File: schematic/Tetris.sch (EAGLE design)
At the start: 16 parts, among them U1 ATTINY45-20P, U2 OLED_0.96_I2C, X1 Batt

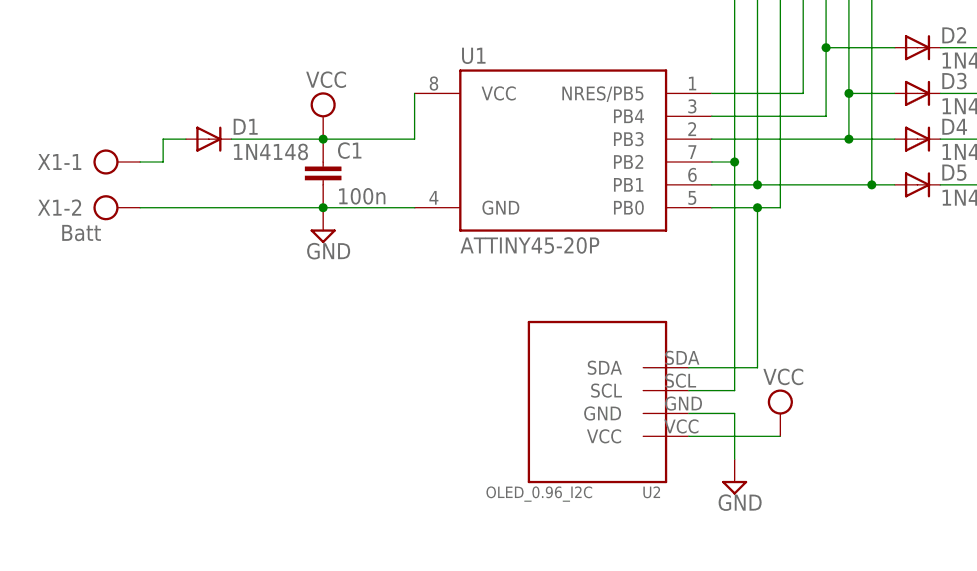
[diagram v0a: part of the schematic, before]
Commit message: Add files via upload
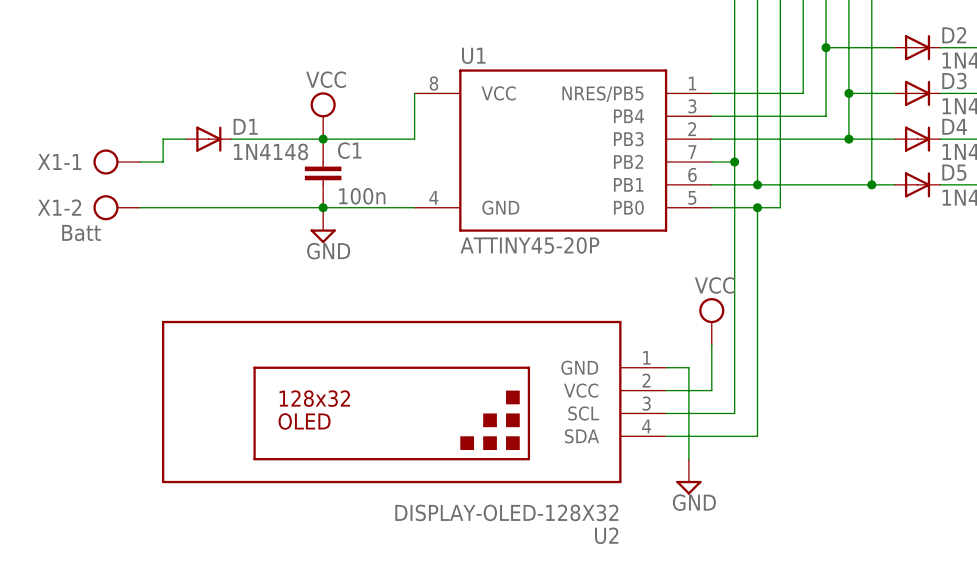
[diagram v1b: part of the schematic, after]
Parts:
- U2: value OLED_0.96_I2C -> DISPLAY-OLED-128X32; device tft_1_8_1_44_oled_0_96:OLED_0.96_I2C -> diy-modules:DISPLAY-OLED-128X32
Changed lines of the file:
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@@
 <parts>
 <part name="JP1" library="avr-7" deviceset="AVR-ISP-10" device=""/>
-<part name="U2" library="tft_1_8_1_44_oled_0_96" deviceset="OLED_0.96_I2C" device=""/>
 <part name="S1" library="switch-omron" deviceset="10-XX" device="" value="A"/>
 <part name="S2" library="switch-omron" deviceset="10-XX" device="" value="Up"/>
@@
 <part name="SUPPLY5" library="supply2" deviceset="VCC" device=""/>
 <part name="SUPPLY6" library="supply2" deviceset="VCC" device=""/>
+<part name="U2" library="diy-modules" deviceset="DISPLAY-OLED-128X32" device=""/>
 </parts>
 <sheets>
@@
 <instances>
 <instance part="JP1" gate="G$1" x="68.58" y="68.58"/>
-<instance part="U2" gate="G$1" x="68.58" y="10.16" rot="R90"/>
 <instance part="S1" gate="1" x="132.08" y="50.8" rot="R270"/>
 <instance part="S2" gate="1" x="149.86" y="50.8" rot="R270"/>
@@
 <instance part="SUPPLY1" gate="GND" x="58.42" y="58.42"/>
 <instance part="SUPPLY2" gate="GND" x="38.1" y="27.94"/>
-<instance part="SUPPLY3" gate="GND" x="83.82" y="0"/>
-<instance part="SUPPLY4" gate="G$1" x="88.9" y="7.62"/>
+<instance part="SUPPLY3" gate="GND" x="78.74" y="0"/>
+<instance part="SUPPLY4" gate="G$1" x="81.28" y="17.78"/>
 <instance part="SUPPLY5" gate="G$1" x="38.1" y="40.64"/>
 <instance part="SUPPLY6" gate="G$1" x="83.82" y="76.2"/>
+<instance part="U2" gate="G$1" x="45.72" y="7.62" rot="R180"/>
 </instances>
 <busses>
@@
 <pinref part="U1" gate="G$1" pin="PB0"/>
 <wire x1="81.28" y1="30.48" x2="86.36" y2="30.48" width="0.1524" layer="91"/>
+<wire x1="86.36" y1="30.48" x2="88.9" y2="30.48" width="0.1524" layer="91"/>
+<wire x1="86.36" y1="5.08" x2="86.36" y2="30.48" width="0.1524" layer="91"/>
+<junction x="86.36" y="30.48"/>
 <pinref part="U2" gate="G$1" pin="SDA"/>
-<wire x1="86.36" y1="30.48" x2="88.9" y2="30.48" width="0.1524" layer="91"/>
-<wire x1="78.74" y1="12.7" x2="86.36" y2="12.7" width="0.1524" layer="91"/>
-<wire x1="86.36" y1="12.7" x2="86.36" y2="30.48" width="0.1524" layer="91"/>
-<junction x="86.36" y="30.48"/>
+<wire x1="76.2" y1="5.08" x2="86.36" y2="5.08" width="0.1524" layer="91"/>
 </segment>
 </net>
@@
 <pinref part="JP1" gate="G$1" pin="7"/>
 <wire x1="83.82" y1="63.5" x2="73.66" y2="63.5" width="0.1524" layer="91"/>
+<wire x1="83.82" y1="7.62" x2="83.82" y2="35.56" width="0.1524" layer="91"/>
+<junction x="83.82" y="35.56"/>
 <pinref part="U2" gate="G$1" pin="SCL"/>
-<wire x1="78.74" y1="10.16" x2="83.82" y2="10.16" width="0.1524" layer="91"/>
-<wire x1="83.82" y1="10.16" x2="83.82" y2="35.56" width="0.1524" layer="91"/>
-<junction x="83.82" y="35.56"/>
+<wire x1="76.2" y1="7.62" x2="83.82" y2="7.62" width="0.1524" layer="91"/>
 </segment>
 </net>
@@
 </segment>
 <segment>
+<pinref part="U2" gate="G$1" pin="GND"/>
 <pinref part="SUPPLY3" gate="GND" pin="GND"/>
-<wire x1="83.82" y1="2.54" x2="83.82" y2="7.62" width="0.1524" layer="91"/>
-<pinref part="U2" gate="G$1" pin="GND"/>
-<wire x1="83.82" y1="7.62" x2="78.74" y2="7.62" width="0.1524" layer="91"/>
+<wire x1="76.2" y1="12.7" x2="78.74" y2="12.7" width="0.1524" layer="91"/>
+<wire x1="78.74" y1="12.7" x2="78.74" y2="2.54" width="0.1524" layer="91"/>
 </segment>
 </net>
@@
 </segment>
 <segment>
+<pinref part="U2" gate="G$1" pin="VCC"/>
 <pinref part="SUPPLY4" gate="G$1" pin="VCC"/>
-<pinref part="U2" gate="G$1" pin="VCC"/>
-<wire x1="88.9" y1="5.08" x2="78.74" y2="5.08" width="0.1524" layer="91"/>
-</segment>
-</net>
+<wire x1="76.2" y1="10.16" x2="81.28" y2="10.16" width="0.1524" layer="91"/>
+<wire x1="81.28" y1="10.16" x2="81.28" y2="15.24" width="0.1524" layer="91"/>
+</segment>
+</net>
